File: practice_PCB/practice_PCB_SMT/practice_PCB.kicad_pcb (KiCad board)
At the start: 2 copper layers, 24.4 x 24.1 mm, 23 parts, among them J1 5V, J2 GND

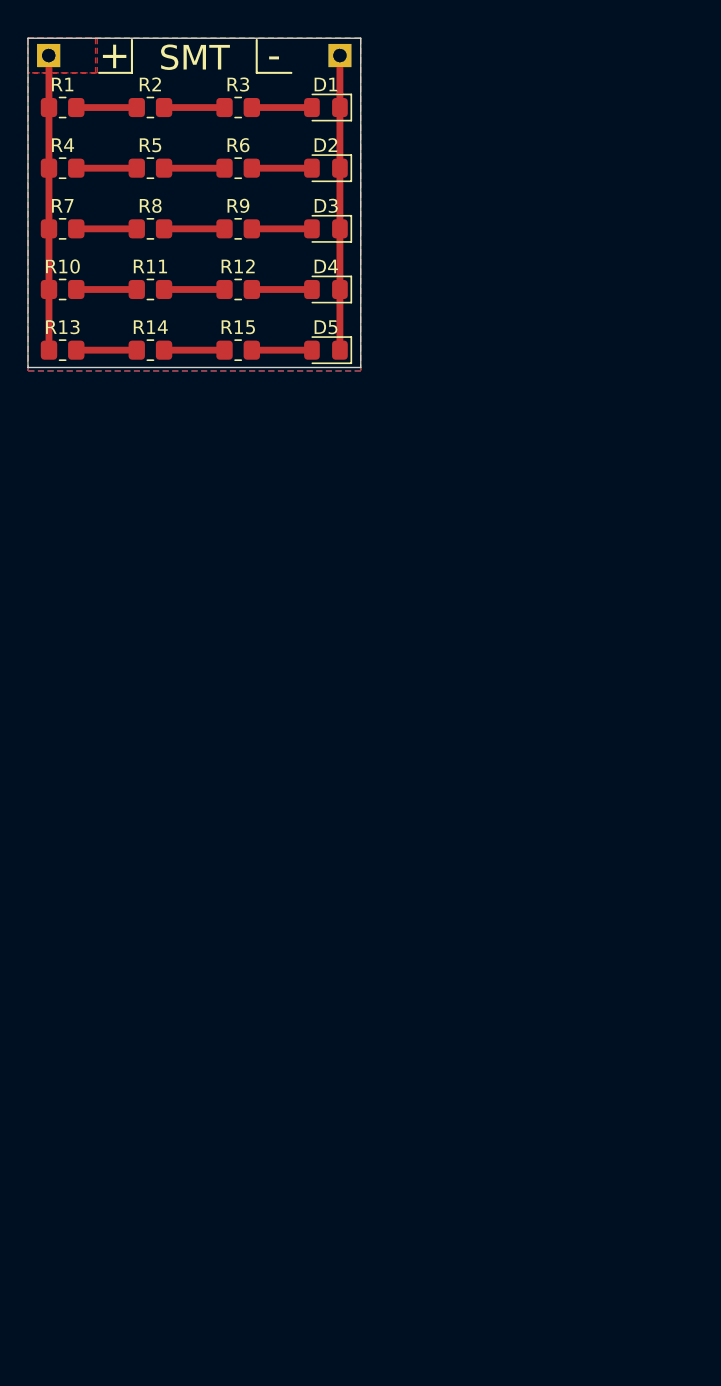
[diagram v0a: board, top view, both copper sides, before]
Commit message: make an array
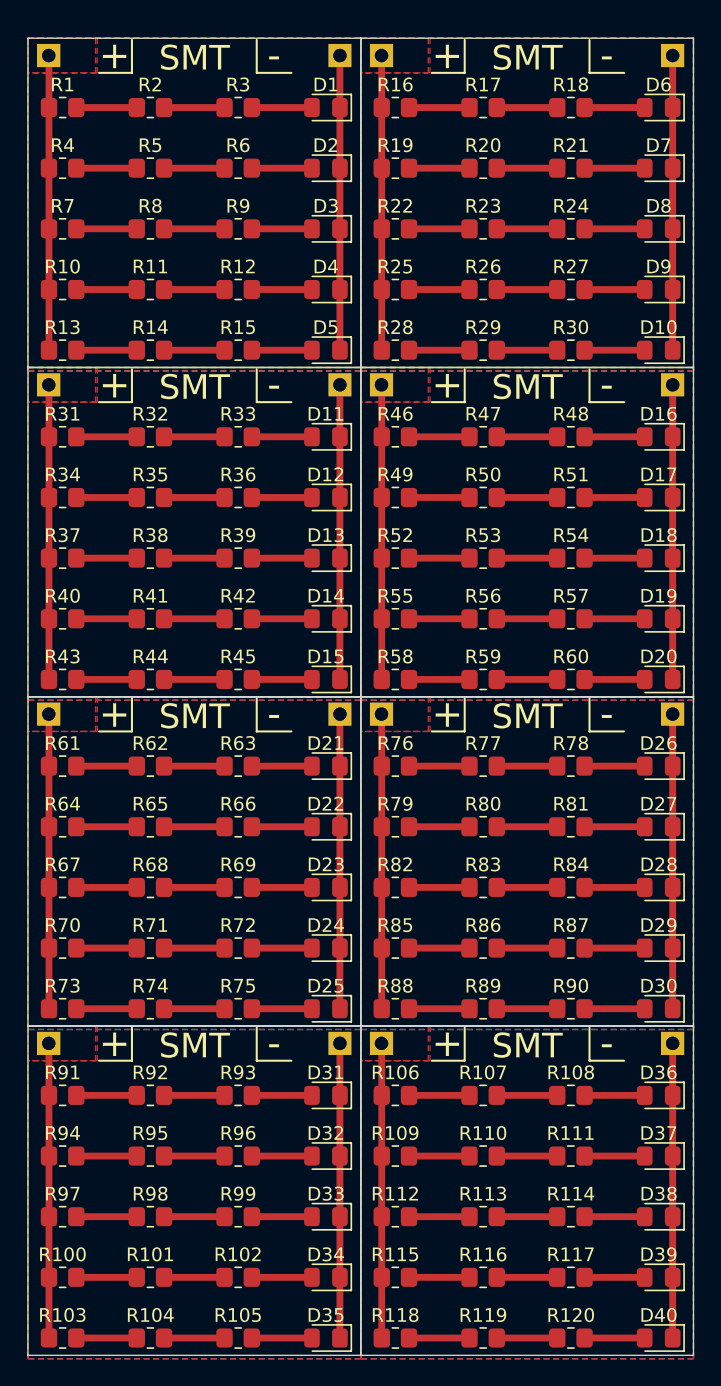
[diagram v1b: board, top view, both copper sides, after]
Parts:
- added D10: LED, LED_SMD:LED_0805_2012Metric_Pad1.15x1.40mm_HandSolder, F.Cu at (183.4, 88.9)
- added D11: LED, LED_SMD:LED_0805_2012Metric_Pad1.15x1.40mm_HandSolder, F.Cu at (159.0, 95.2)
- added D12: LED, LED_SMD:LED_0805_2012Metric_Pad1.15x1.40mm_HandSolder, F.Cu at (159.0, 99.7)
- added D13: LED, LED_SMD:LED_0805_2012Metric_Pad1.15x1.40mm_HandSolder, F.Cu at (159.0, 104.1)
- added D14: LED, LED_SMD:LED_0805_2012Metric_Pad1.15x1.40mm_HandSolder, F.Cu at (159.0, 108.6)
- added D15: LED, LED_SMD:LED_0805_2012Metric_Pad1.15x1.40mm_HandSolder, F.Cu at (159.0, 113.0)
- added D16: LED, LED_SMD:LED_0805_2012Metric_Pad1.15x1.40mm_HandSolder, F.Cu at (183.4, 95.2)
- added D17: LED, LED_SMD:LED_0805_2012Metric_Pad1.15x1.40mm_HandSolder, F.Cu at (183.4, 99.7)
- added D18: LED, LED_SMD:LED_0805_2012Metric_Pad1.15x1.40mm_HandSolder, F.Cu at (183.4, 104.1)
- added D19: LED, LED_SMD:LED_0805_2012Metric_Pad1.15x1.40mm_HandSolder, F.Cu at (183.4, 108.6)
- added D20: LED, LED_SMD:LED_0805_2012Metric_Pad1.15x1.40mm_HandSolder, F.Cu at (183.4, 113.0)
- added D21: LED, LED_SMD:LED_0805_2012Metric_Pad1.15x1.40mm_HandSolder, F.Cu at (159.0, 119.4)
- added D22: LED, LED_SMD:LED_0805_2012Metric_Pad1.15x1.40mm_HandSolder, F.Cu at (159.0, 123.8)
- added D23: LED, LED_SMD:LED_0805_2012Metric_Pad1.15x1.40mm_HandSolder, F.Cu at (159.0, 128.3)
- added D24: LED, LED_SMD:LED_0805_2012Metric_Pad1.15x1.40mm_HandSolder, F.Cu at (159.0, 132.7)
- added D25: LED, LED_SMD:LED_0805_2012Metric_Pad1.15x1.40mm_HandSolder, F.Cu at (159.0, 137.2)
- added D26: LED, LED_SMD:LED_0805_2012Metric_Pad1.15x1.40mm_HandSolder, F.Cu at (183.4, 119.4)
- added D27: LED, LED_SMD:LED_0805_2012Metric_Pad1.15x1.40mm_HandSolder, F.Cu at (183.4, 123.8)
- added D28: LED, LED_SMD:LED_0805_2012Metric_Pad1.15x1.40mm_HandSolder, F.Cu at (183.4, 128.3)
- added D29: LED, LED_SMD:LED_0805_2012Metric_Pad1.15x1.40mm_HandSolder, F.Cu at (183.4, 132.7)
- added D30: LED, LED_SMD:LED_0805_2012Metric_Pad1.15x1.40mm_HandSolder, F.Cu at (183.4, 137.2)
- added D31: LED, LED_SMD:LED_0805_2012Metric_Pad1.15x1.40mm_HandSolder, F.Cu at (159.0, 143.5)
- added D32: LED, LED_SMD:LED_0805_2012Metric_Pad1.15x1.40mm_HandSolder, F.Cu at (159.0, 148.0)
- added D33: LED, LED_SMD:LED_0805_2012Metric_Pad1.15x1.40mm_HandSolder, F.Cu at (159.0, 152.4)
- added D34: LED, LED_SMD:LED_0805_2012Metric_Pad1.15x1.40mm_HandSolder, F.Cu at (159.0, 156.8)
- added D35: LED, LED_SMD:LED_0805_2012Metric_Pad1.15x1.40mm_HandSolder, F.Cu at (159.0, 161.3)
- added D36: LED, LED_SMD:LED_0805_2012Metric_Pad1.15x1.40mm_HandSolder, F.Cu at (183.4, 143.5)
- added D37: LED, LED_SMD:LED_0805_2012Metric_Pad1.15x1.40mm_HandSolder, F.Cu at (183.4, 148.0)
- added D38: LED, LED_SMD:LED_0805_2012Metric_Pad1.15x1.40mm_HandSolder, F.Cu at (183.4, 152.4)
- added D39: LED, LED_SMD:LED_0805_2012Metric_Pad1.15x1.40mm_HandSolder, F.Cu at (183.4, 156.8)
- added D40: LED, LED_SMD:LED_0805_2012Metric_Pad1.15x1.40mm_HandSolder, F.Cu at (183.4, 161.3)
- added D6: LED, LED_SMD:LED_0805_2012Metric_Pad1.15x1.40mm_HandSolder, F.Cu at (183.4, 71.1)
- added D7: LED, LED_SMD:LED_0805_2012Metric_Pad1.15x1.40mm_HandSolder, F.Cu at (183.4, 75.6)
- added D8: LED, LED_SMD:LED_0805_2012Metric_Pad1.15x1.40mm_HandSolder, F.Cu at (183.4, 80.0)
- added D9: LED, LED_SMD:LED_0805_2012Metric_Pad1.15x1.40mm_HandSolder, F.Cu at (183.4, 84.5)
- added G***1: LOGO, practice_PCB:MWG, B.Cu at (181.4, 86.4)
- added G***2: LOGO, practice_PCB:MWG, B.Cu at (157.0, 110.5)
- added G***3: LOGO, practice_PCB:MWG, B.Cu at (181.4, 110.5)
- added G***4: LOGO, practice_PCB:MWG, B.Cu at (157.0, 134.6)
- added G***5: LOGO, practice_PCB:MWG, B.Cu at (181.4, 134.6)
- added G***6: LOGO, practice_PCB:MWG, B.Cu at (157.0, 158.8)
- added G***7: LOGO, practice_PCB:MWG, B.Cu at (181.4, 158.8)
- added J10: GND, practice_PCB:PinSocket_1x01_P2.54mm_Vertical, F.Cu at (160.0, 115.6)
- added J11: 5V, practice_PCB:PinSocket_1x01_P2.54mm_Vertical, F.Cu at (163.1, 115.6)
- added J12: GND, practice_PCB:PinSocket_1x01_P2.54mm_Vertical, F.Cu at (184.4, 115.6)
- added J13: 5V, practice_PCB:PinSocket_1x01_P2.54mm_Vertical, F.Cu at (138.7, 139.7)
- added J14: GND, practice_PCB:PinSocket_1x01_P2.54mm_Vertical, F.Cu at (160.0, 139.7)
- added J15: 5V, practice_PCB:PinSocket_1x01_P2.54mm_Vertical, F.Cu at (163.1, 139.7)
- added J16: GND, practice_PCB:PinSocket_1x01_P2.54mm_Vertical, F.Cu at (184.4, 139.7)
- added J3: 5V, practice_PCB:PinSocket_1x01_P2.54mm_Vertical, F.Cu at (163.1, 67.3)
- added J4: GND, practice_PCB:PinSocket_1x01_P2.54mm_Vertical, F.Cu at (184.4, 67.3)
- added J5: 5V, practice_PCB:PinSocket_1x01_P2.54mm_Vertical, F.Cu at (138.7, 91.4)
- added J6: GND, practice_PCB:PinSocket_1x01_P2.54mm_Vertical, F.Cu at (160.0, 91.4)
- added J7: 5V, practice_PCB:PinSocket_1x01_P2.54mm_Vertical, F.Cu at (163.1, 91.4)
- added J8: GND, practice_PCB:PinSocket_1x01_P2.54mm_Vertical, F.Cu at (184.4, 91.4)
- added J9: 5V, practice_PCB:PinSocket_1x01_P2.54mm_Vertical, F.Cu at (138.7, 115.6)
- added R100: 60, Resistor_SMD:R_0805_2012Metric_Pad1.20x1.40mm_HandSolder, F.Cu at (139.7, 156.8)
- added R101: 60, Resistor_SMD:R_0805_2012Metric_Pad1.20x1.40mm_HandSolder, F.Cu at (146.1, 156.8)
- added R102: 60, Resistor_SMD:R_0805_2012Metric_Pad1.20x1.40mm_HandSolder, F.Cu at (152.6, 156.8)
- added R103: 60, Resistor_SMD:R_0805_2012Metric_Pad1.20x1.40mm_HandSolder, F.Cu at (139.7, 161.3)
- added R104: 60, Resistor_SMD:R_0805_2012Metric_Pad1.20x1.40mm_HandSolder, F.Cu at (146.1, 161.3)
- added R105: 60, Resistor_SMD:R_0805_2012Metric_Pad1.20x1.40mm_HandSolder, F.Cu at (152.6, 161.3)
- added R106: 60, Resistor_SMD:R_0805_2012Metric_Pad1.20x1.40mm_HandSolder, F.Cu at (164.1, 143.5)
- added R107: 60, Resistor_SMD:R_0805_2012Metric_Pad1.20x1.40mm_HandSolder, F.Cu at (170.5, 143.5)
- added R108: 60, Resistor_SMD:R_0805_2012Metric_Pad1.20x1.40mm_HandSolder, F.Cu at (176.9, 143.5)
- added R109: 60, Resistor_SMD:R_0805_2012Metric_Pad1.20x1.40mm_HandSolder, F.Cu at (164.1, 148.0)
- added R110: 60, Resistor_SMD:R_0805_2012Metric_Pad1.20x1.40mm_HandSolder, F.Cu at (170.5, 148.0)
- added R111: 60, Resistor_SMD:R_0805_2012Metric_Pad1.20x1.40mm_HandSolder, F.Cu at (176.9, 148.0)
- added R112: 60, Resistor_SMD:R_0805_2012Metric_Pad1.20x1.40mm_HandSolder, F.Cu at (164.1, 152.4)
- added R113: 60, Resistor_SMD:R_0805_2012Metric_Pad1.20x1.40mm_HandSolder, F.Cu at (170.5, 152.4)
- added R114: 60, Resistor_SMD:R_0805_2012Metric_Pad1.20x1.40mm_HandSolder, F.Cu at (176.9, 152.4)
- added R115: 60, Resistor_SMD:R_0805_2012Metric_Pad1.20x1.40mm_HandSolder, F.Cu at (164.1, 156.8)
- added R116: 60, Resistor_SMD:R_0805_2012Metric_Pad1.20x1.40mm_HandSolder, F.Cu at (170.5, 156.8)
- added R117: 60, Resistor_SMD:R_0805_2012Metric_Pad1.20x1.40mm_HandSolder, F.Cu at (176.9, 156.8)
- added R118: 60, Resistor_SMD:R_0805_2012Metric_Pad1.20x1.40mm_HandSolder, F.Cu at (164.1, 161.3)
- added R119: 60, Resistor_SMD:R_0805_2012Metric_Pad1.20x1.40mm_HandSolder, F.Cu at (170.5, 161.3)
- added R120: 60, Resistor_SMD:R_0805_2012Metric_Pad1.20x1.40mm_HandSolder, F.Cu at (176.9, 161.3)
- added R16: 60, Resistor_SMD:R_0805_2012Metric_Pad1.20x1.40mm_HandSolder, F.Cu at (164.1, 71.1)
- added R17: 60, Resistor_SMD:R_0805_2012Metric_Pad1.20x1.40mm_HandSolder, F.Cu at (170.5, 71.1)
- added R18: 60, Resistor_SMD:R_0805_2012Metric_Pad1.20x1.40mm_HandSolder, F.Cu at (176.9, 71.1)
- added R19: 60, Resistor_SMD:R_0805_2012Metric_Pad1.20x1.40mm_HandSolder, F.Cu at (164.1, 75.6)
- added R20: 60, Resistor_SMD:R_0805_2012Metric_Pad1.20x1.40mm_HandSolder, F.Cu at (170.5, 75.6)
- added R21: 60, Resistor_SMD:R_0805_2012Metric_Pad1.20x1.40mm_HandSolder, F.Cu at (176.9, 75.6)
- added R22: 60, Resistor_SMD:R_0805_2012Metric_Pad1.20x1.40mm_HandSolder, F.Cu at (164.1, 80.0)
- added R23: 60, Resistor_SMD:R_0805_2012Metric_Pad1.20x1.40mm_HandSolder, F.Cu at (170.5, 80.0)
- added R24: 60, Resistor_SMD:R_0805_2012Metric_Pad1.20x1.40mm_HandSolder, F.Cu at (176.9, 80.0)
- added R25: 60, Resistor_SMD:R_0805_2012Metric_Pad1.20x1.40mm_HandSolder, F.Cu at (164.1, 84.5)
- added R26: 60, Resistor_SMD:R_0805_2012Metric_Pad1.20x1.40mm_HandSolder, F.Cu at (170.5, 84.5)
- added R27: 60, Resistor_SMD:R_0805_2012Metric_Pad1.20x1.40mm_HandSolder, F.Cu at (176.9, 84.5)
- added R28: 60, Resistor_SMD:R_0805_2012Metric_Pad1.20x1.40mm_HandSolder, F.Cu at (164.1, 88.9)
- added R29: 60, Resistor_SMD:R_0805_2012Metric_Pad1.20x1.40mm_HandSolder, F.Cu at (170.5, 88.9)
- added R30: 60, Resistor_SMD:R_0805_2012Metric_Pad1.20x1.40mm_HandSolder, F.Cu at (176.9, 88.9)
- added R31: 60, Resistor_SMD:R_0805_2012Metric_Pad1.20x1.40mm_HandSolder, F.Cu at (139.7, 95.2)
- added R32: 60, Resistor_SMD:R_0805_2012Metric_Pad1.20x1.40mm_HandSolder, F.Cu at (146.1, 95.2)
- added R33: 60, Resistor_SMD:R_0805_2012Metric_Pad1.20x1.40mm_HandSolder, F.Cu at (152.6, 95.2)
- added R34: 60, Resistor_SMD:R_0805_2012Metric_Pad1.20x1.40mm_HandSolder, F.Cu at (139.7, 99.7)
- added R35: 60, Resistor_SMD:R_0805_2012Metric_Pad1.20x1.40mm_HandSolder, F.Cu at (146.1, 99.7)
- added R36: 60, Resistor_SMD:R_0805_2012Metric_Pad1.20x1.40mm_HandSolder, F.Cu at (152.6, 99.7)
- added R37: 60, Resistor_SMD:R_0805_2012Metric_Pad1.20x1.40mm_HandSolder, F.Cu at (139.7, 104.1)
- added R38: 60, Resistor_SMD:R_0805_2012Metric_Pad1.20x1.40mm_HandSolder, F.Cu at (146.1, 104.1)
- added R39: 60, Resistor_SMD:R_0805_2012Metric_Pad1.20x1.40mm_HandSolder, F.Cu at (152.6, 104.1)
- added R40: 60, Resistor_SMD:R_0805_2012Metric_Pad1.20x1.40mm_HandSolder, F.Cu at (139.7, 108.6)
- added R41: 60, Resistor_SMD:R_0805_2012Metric_Pad1.20x1.40mm_HandSolder, F.Cu at (146.1, 108.6)
- added R42: 60, Resistor_SMD:R_0805_2012Metric_Pad1.20x1.40mm_HandSolder, F.Cu at (152.6, 108.6)
- added R43: 60, Resistor_SMD:R_0805_2012Metric_Pad1.20x1.40mm_HandSolder, F.Cu at (139.7, 113.0)
- added R44: 60, Resistor_SMD:R_0805_2012Metric_Pad1.20x1.40mm_HandSolder, F.Cu at (146.1, 113.0)
- added R45: 60, Resistor_SMD:R_0805_2012Metric_Pad1.20x1.40mm_HandSolder, F.Cu at (152.6, 113.0)
- added R46: 60, Resistor_SMD:R_0805_2012Metric_Pad1.20x1.40mm_HandSolder, F.Cu at (164.1, 95.2)
- added R47: 60, Resistor_SMD:R_0805_2012Metric_Pad1.20x1.40mm_HandSolder, F.Cu at (170.5, 95.2)
- added R48: 60, Resistor_SMD:R_0805_2012Metric_Pad1.20x1.40mm_HandSolder, F.Cu at (176.9, 95.2)
- added R49: 60, Resistor_SMD:R_0805_2012Metric_Pad1.20x1.40mm_HandSolder, F.Cu at (164.1, 99.7)
- added R50: 60, Resistor_SMD:R_0805_2012Metric_Pad1.20x1.40mm_HandSolder, F.Cu at (170.5, 99.7)
- added R51: 60, Resistor_SMD:R_0805_2012Metric_Pad1.20x1.40mm_HandSolder, F.Cu at (176.9, 99.7)
- added R52: 60, Resistor_SMD:R_0805_2012Metric_Pad1.20x1.40mm_HandSolder, F.Cu at (164.1, 104.1)
- added R53: 60, Resistor_SMD:R_0805_2012Metric_Pad1.20x1.40mm_HandSolder, F.Cu at (170.5, 104.1)
- added R54: 60, Resistor_SMD:R_0805_2012Metric_Pad1.20x1.40mm_HandSolder, F.Cu at (176.9, 104.1)
- added R55: 60, Resistor_SMD:R_0805_2012Metric_Pad1.20x1.40mm_HandSolder, F.Cu at (164.1, 108.6)
- added R56: 60, Resistor_SMD:R_0805_2012Metric_Pad1.20x1.40mm_HandSolder, F.Cu at (170.5, 108.6)
- added R57: 60, Resistor_SMD:R_0805_2012Metric_Pad1.20x1.40mm_HandSolder, F.Cu at (176.9, 108.6)
- added R58: 60, Resistor_SMD:R_0805_2012Metric_Pad1.20x1.40mm_HandSolder, F.Cu at (164.1, 113.0)
- added R59: 60, Resistor_SMD:R_0805_2012Metric_Pad1.20x1.40mm_HandSolder, F.Cu at (170.5, 113.0)
- added R60: 60, Resistor_SMD:R_0805_2012Metric_Pad1.20x1.40mm_HandSolder, F.Cu at (176.9, 113.0)
- added R61: 60, Resistor_SMD:R_0805_2012Metric_Pad1.20x1.40mm_HandSolder, F.Cu at (139.7, 119.4)
- added R62: 60, Resistor_SMD:R_0805_2012Metric_Pad1.20x1.40mm_HandSolder, F.Cu at (146.1, 119.4)
- added R63: 60, Resistor_SMD:R_0805_2012Metric_Pad1.20x1.40mm_HandSolder, F.Cu at (152.6, 119.4)
- added R64: 60, Resistor_SMD:R_0805_2012Metric_Pad1.20x1.40mm_HandSolder, F.Cu at (139.7, 123.8)
- added R65: 60, Resistor_SMD:R_0805_2012Metric_Pad1.20x1.40mm_HandSolder, F.Cu at (146.1, 123.8)
- added R66: 60, Resistor_SMD:R_0805_2012Metric_Pad1.20x1.40mm_HandSolder, F.Cu at (152.6, 123.8)
- added R67: 60, Resistor_SMD:R_0805_2012Metric_Pad1.20x1.40mm_HandSolder, F.Cu at (139.7, 128.3)
- added R68: 60, Resistor_SMD:R_0805_2012Metric_Pad1.20x1.40mm_HandSolder, F.Cu at (146.1, 128.3)
- added R69: 60, Resistor_SMD:R_0805_2012Metric_Pad1.20x1.40mm_HandSolder, F.Cu at (152.6, 128.3)
- added R70: 60, Resistor_SMD:R_0805_2012Metric_Pad1.20x1.40mm_HandSolder, F.Cu at (139.7, 132.7)
- added R71: 60, Resistor_SMD:R_0805_2012Metric_Pad1.20x1.40mm_HandSolder, F.Cu at (146.1, 132.7)
- added R72: 60, Resistor_SMD:R_0805_2012Metric_Pad1.20x1.40mm_HandSolder, F.Cu at (152.6, 132.7)
- added R73: 60, Resistor_SMD:R_0805_2012Metric_Pad1.20x1.40mm_HandSolder, F.Cu at (139.7, 137.2)
- added R74: 60, Resistor_SMD:R_0805_2012Metric_Pad1.20x1.40mm_HandSolder, F.Cu at (146.1, 137.2)
- added R75: 60, Resistor_SMD:R_0805_2012Metric_Pad1.20x1.40mm_HandSolder, F.Cu at (152.6, 137.2)
- added R76: 60, Resistor_SMD:R_0805_2012Metric_Pad1.20x1.40mm_HandSolder, F.Cu at (164.1, 119.4)
- added R77: 60, Resistor_SMD:R_0805_2012Metric_Pad1.20x1.40mm_HandSolder, F.Cu at (170.5, 119.4)
- added R78: 60, Resistor_SMD:R_0805_2012Metric_Pad1.20x1.40mm_HandSolder, F.Cu at (176.9, 119.4)
- added R79: 60, Resistor_SMD:R_0805_2012Metric_Pad1.20x1.40mm_HandSolder, F.Cu at (164.1, 123.8)
- added R80: 60, Resistor_SMD:R_0805_2012Metric_Pad1.20x1.40mm_HandSolder, F.Cu at (170.5, 123.8)
- added R81: 60, Resistor_SMD:R_0805_2012Metric_Pad1.20x1.40mm_HandSolder, F.Cu at (176.9, 123.8)
- added R82: 60, Resistor_SMD:R_0805_2012Metric_Pad1.20x1.40mm_HandSolder, F.Cu at (164.1, 128.3)
- added R83: 60, Resistor_SMD:R_0805_2012Metric_Pad1.20x1.40mm_HandSolder, F.Cu at (170.5, 128.3)
- added R84: 60, Resistor_SMD:R_0805_2012Metric_Pad1.20x1.40mm_HandSolder, F.Cu at (176.9, 128.3)
- added R85: 60, Resistor_SMD:R_0805_2012Metric_Pad1.20x1.40mm_HandSolder, F.Cu at (164.1, 132.7)
- added R86: 60, Resistor_SMD:R_0805_2012Metric_Pad1.20x1.40mm_HandSolder, F.Cu at (170.5, 132.7)
- added R87: 60, Resistor_SMD:R_0805_2012Metric_Pad1.20x1.40mm_HandSolder, F.Cu at (176.9, 132.7)
- added R88: 60, Resistor_SMD:R_0805_2012Metric_Pad1.20x1.40mm_HandSolder, F.Cu at (164.1, 137.2)
- added R89: 60, Resistor_SMD:R_0805_2012Metric_Pad1.20x1.40mm_HandSolder, F.Cu at (170.5, 137.2)
- added R90: 60, Resistor_SMD:R_0805_2012Metric_Pad1.20x1.40mm_HandSolder, F.Cu at (176.9, 137.2)
- added R91: 60, Resistor_SMD:R_0805_2012Metric_Pad1.20x1.40mm_HandSolder, F.Cu at (139.7, 143.5)
- added R92: 60, Resistor_SMD:R_0805_2012Metric_Pad1.20x1.40mm_HandSolder, F.Cu at (146.1, 143.5)
- added R93: 60, Resistor_SMD:R_0805_2012Metric_Pad1.20x1.40mm_HandSolder, F.Cu at (152.6, 143.5)
- added R94: 60, Resistor_SMD:R_0805_2012Metric_Pad1.20x1.40mm_HandSolder, F.Cu at (139.7, 148.0)
- added R95: 60, Resistor_SMD:R_0805_2012Metric_Pad1.20x1.40mm_HandSolder, F.Cu at (146.1, 148.0)
- added R96: 60, Resistor_SMD:R_0805_2012Metric_Pad1.20x1.40mm_HandSolder, F.Cu at (152.6, 148.0)
- added R97: 60, Resistor_SMD:R_0805_2012Metric_Pad1.20x1.40mm_HandSolder, F.Cu at (139.7, 152.4)
- added R98: 60, Resistor_SMD:R_0805_2012Metric_Pad1.20x1.40mm_HandSolder, F.Cu at (146.1, 152.4)
- added R99: 60, Resistor_SMD:R_0805_2012Metric_Pad1.20x1.40mm_HandSolder, F.Cu at (152.6, 152.4)
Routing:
- net +5V: track 21.6 -> 172.8 mm
- net GND: track 21.6 -> 172.7 mm
- net Net-(R7-Pad2): track 4.43 -> 35.5 mm
- net Net-(R4-Pad2): track 4.43 -> 35.5 mm
- net Net-(R13-Pad2): track 4.43 -> 35.5 mm
- net Net-(R10-Pad2): track 4.43 -> 35.5 mm
- net Net-(R1-Pad2): track 4.43 -> 35.5 mm
- net Net-(R8-Pad2): track 4.43 -> 35.5 mm
- net Net-(R5-Pad2): track 4.43 -> 35.5 mm
- net Net-(R2-Pad2): track 4.43 -> 35.5 mm
- net Net-(R14-Pad2): track 4.43 -> 35.5 mm
- net Net-(R11-Pad2): track 4.43 -> 35.5 mm
- net Net-(D5-Pad2): track 4.41 -> 35.3 mm
- net Net-(D4-Pad2): track 4.41 -> 35.3 mm
- net Net-(D3-Pad2): track 4.41 -> 35.3 mm
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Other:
- board size 24.4 x 24.1 mm -> 48.8 x 96.5 mm
